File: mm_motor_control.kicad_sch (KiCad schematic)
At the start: 11 parts, among them U3 STSPIN240

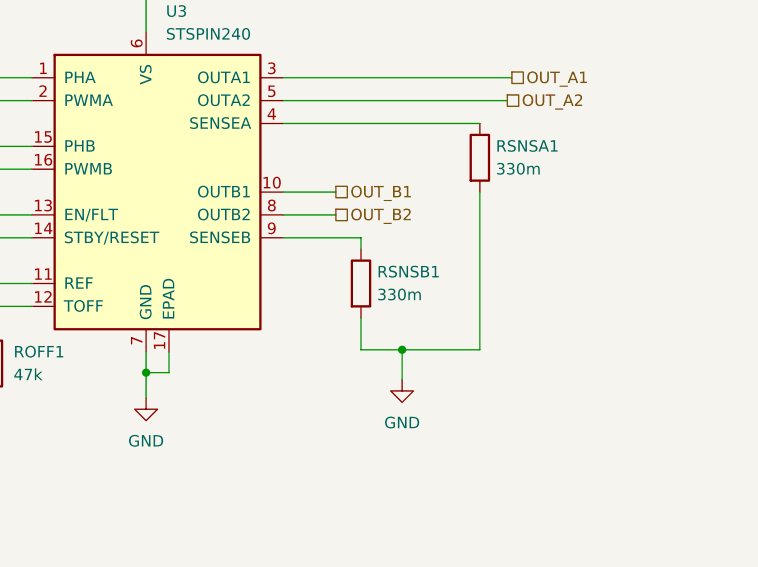
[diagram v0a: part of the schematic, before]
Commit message: fin de TP4
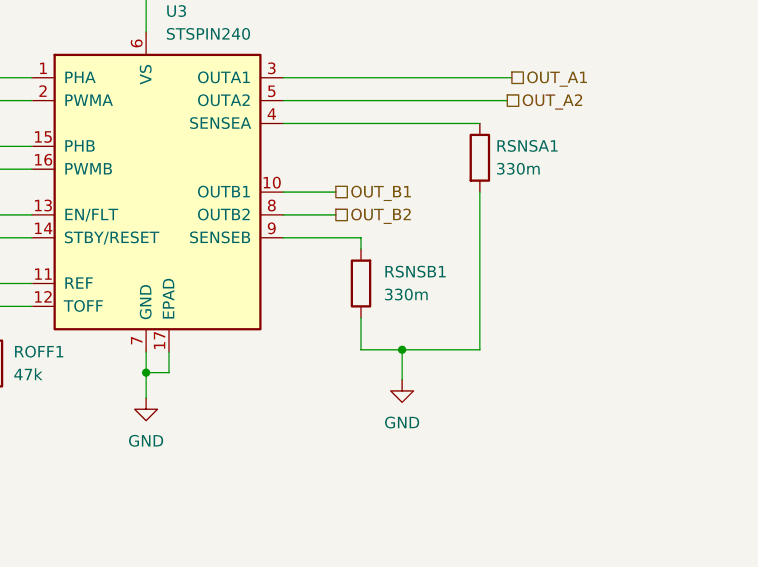
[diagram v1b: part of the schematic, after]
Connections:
- net GND: now also RSNSB1.1; no longer RSNSB1.2
- net at U3.9 (SENSEB): now also RSNSB1.2; no longer RSNSB1.1
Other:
- moved on the sheet: RSNSB1
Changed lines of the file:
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@@
     )
   )
-  (symbol (lib_id "Device:R") (at 167.64 100.33 0) (unit 1)
+  (symbol (lib_id "Device:R") (at 167.64 100.33 180) (unit 1)
     (in_bom yes) (on_board yes) (dnp no) (fields_autoplaced)
-    (property "Reference" "RSNSB1" (at 169.418 99.06 0)
-      (effects (font (size 1.27 1.27)) (justify left))
+    (property "Reference" "RSNSB1" (at 170.18 99.06 0)
+      (effects (font (size 1.27 1.27)) (justify right))
     )
-    (property "Value" "330m" (at 169.418 101.6 0)
-      (effects (font (size 1.27 1.27)) (justify left))
+    (property "Value" "330m" (at 170.18 101.6 0)
+      (effects (font (size 1.27 1.27)) (justify right))
     )
-    (property "Footprint" "Resistor_SMD:R_0603_1608Metric" (at 165.862 100.33 90)
+    (property "Footprint" "Resistor_SMD:R_0603_1608Metric" (at 169.418 100.33 90)
       (effects (font (size 1.27 1.27)) hide)
     )
